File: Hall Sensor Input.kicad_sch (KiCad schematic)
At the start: 2 parts

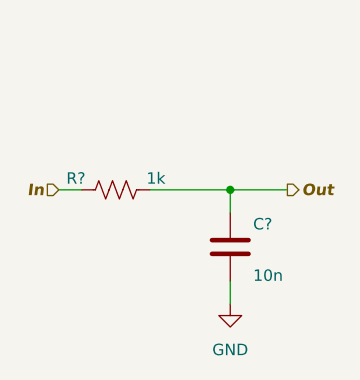
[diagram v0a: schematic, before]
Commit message: Ready for design review
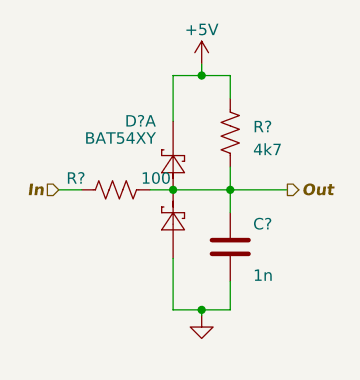
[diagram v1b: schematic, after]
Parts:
- added D?: BAT54XY, Package_TO_SOT_SMD:SOT-363_SC-70-6, symbol Diode:BAT54SW
- added R?: 4k7, Resistor_SMD:R_0402_1005Metric, symbol Device:R_US
- C?: value 10n -> 1n; DigiKey 490-4762-1-ND -> 490-GCM155R71H102KA37JCT-ND; LCSC (none) -> C1852263
- R?: value 1k -> 100; DigiKey 311-1.00KLRCT-ND -> 311-100JRCT-ND; LCSC (none) -> C106233
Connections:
- net GND: now also D?.1 (A)
- net Out: now also D?.6 (COM), R?.2
- new net +5V: D?.2 (K), R?.1

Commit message: Update
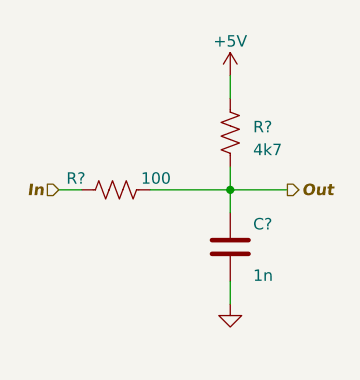
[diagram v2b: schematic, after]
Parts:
- removed D?: BAT54XY, Package_TO_SOT_SMD:SOT-363_SC-70-6, symbol Diode:BAT54SW
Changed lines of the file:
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@@
   (junction (at 146.05 101.6) (diameter 0) (color 0 0 0 0)
   )
-  (junction (at 139.7 101.6) (diameter 0) (color 0 0 0 0)
-  )
-  (junction (at 142.875 114.935) (diameter 0) (color 0 0 0 0)
-  )
-  (junction (at 142.875 88.9) (diameter 0) (color 0 0 0 0)
-  )
-  (wire (pts (xy 139.7 93.98) (xy 139.7 88.9))
-    (stroke (width 0) (type default))
-  )
-  (wire (pts (xy 142.875 114.935) (xy 142.875 115.57))
-    (stroke (width 0) (type default))
-  )
-  (wire (pts (xy 142.875 114.935) (xy 146.05 114.935))
-    (stroke (width 0) (type default))
-  )
-  (wire (pts (xy 146.05 114.935) (xy 146.05 111.76))
-    (stroke (width 0) (type default))
-  )
-  (wire (pts (xy 139.7 114.935) (xy 142.875 114.935))
+  (wire (pts (xy 146.05 114.3) (xy 146.05 111.76))
     (stroke (width 0) (type default))
   )
@@
     (stroke (width 0) (type default))
   )
-  (wire (pts (xy 139.7 109.22) (xy 139.7 114.935))
-    (stroke (width 0) (type default))
-  )
   (wire (pts (xy 146.05 99.06) (xy 146.05 101.6))
     (stroke (width 0) (type default))
   )
-  (wire (pts (xy 142.875 88.9) (xy 146.05 88.9))
-    (stroke (width 0) (type default))
-  )
   (wire (pts (xy 127 101.6) (xy 129.54 101.6))
     (stroke (width 0) (type default))
   )
-  (wire (pts (xy 137.16 101.6) (xy 139.7 101.6))
-    (stroke (width 0) (type default))
-  )
-  (wire (pts (xy 142.875 87.63) (xy 142.875 88.9))
+  (wire (pts (xy 137.16 101.6) (xy 146.05 101.6))
     (stroke (width 0) (type default))
   )
@@
     (stroke (width 0) (type default))
   )
-  (wire (pts (xy 139.7 88.9) (xy 142.875 88.9))
-    (stroke (width 0) (type default))
-  )
   (wire (pts (xy 146.05 88.9) (xy 146.05 91.44))
-    (stroke (width 0) (type default))
-  )
-  (wire (pts (xy 139.7 101.6) (xy 146.05 101.6))
     (stroke (width 0) (type default))
   )
@@
           (reference "C63") (unit 1)
         )
-        (path "/6b38a626-de8c-4b2d-bc76-3a02bc823a86/719c509b-8ff9-4083-837d-a3024db7e531"
-          (reference "C64") (unit 1)
-        )
-      )
-    )
-  )
-  (symbol (lib_id "power:GND") (at 142.875 115.57 0) (unit 1)
+      )
+    )
+  )
+  (symbol (lib_id "power:GND") (at 146.05 114.3 0) (unit 1)
     (in_bom yes) (on_board yes) (dnp no) (fields_autoplaced)
-    (property "Reference" "#PWR02" (at 142.875 121.92 0)
-      (effects (font (size 1.27 1.27)) hide)
-    )
-    (property "Value" "GND" (at 142.875 120.65 0)
-      (effects (font (size 1.27 1.27)) hide)
-    )
-    (property "Footprint" "" (at 142.875 115.57 0)
-      (effects (font (size 1.27 1.27)) hide)
-    )
-    (property "Datasheet" "" (at 142.875 115.57 0)
+    (property "Reference" "#PWR02" (at 146.05 120.65 0)
+      (effects (font (size 1.27 1.27)) hide)
+    )
+    (property "Value" "GND" (at 146.05 119.38 0)
+      (effects (font (size 1.27 1.27)) hide)
+    )
+    (property "Footprint" "" (at 146.05 114.3 0)
+      (effects (font (size 1.27 1.27)) hide)
+    )
+    (property "Datasheet" "" (at 146.05 114.3 0)
       (effects (font (size 1.27 1.27)) hide)
     )
@@
         (path "/6b38a626-de8c-4b2d-bc76-3a02bc823a86/a05ea58c-77e1-4772-b7c7-450b1547e96e"
           (reference "#PWR06") (unit 1)
-        )
-        (path "/6b38a626-de8c-4b2d-bc76-3a02bc823a86/719c509b-8ff9-4083-837d-a3024db7e531"
-          (reference "#PWR08") (unit 1)
         )
       )
@@
           (reference "R?") (unit 1)
         )
-        (path "/6b38a626-de8c-4b2d-bc76-3a02bc823a86/3c576bdf-2a9b-47b5-bf2f-8d65e4282c90"
-          (reference "R?") (unit 1)
-        )
         (path "/6b38a626-de8c-4b2d-bc76-3a02bc823a86/9e0a8a8b-b0ec-4703-8f8c-5ea275317857"
           (reference "R12") (unit 1)
@@
           (reference "R16") (unit 1)
         )
-        (path "/6b38a626-de8c-4b2d-bc76-3a02bc823a86/719c509b-8ff9-4083-837d-a3024db7e531"
-          (reference "R18") (unit 1)
-        )
-      )
-    )
-  )
-  (symbol (lib_id "Diode:BAT54SW") (at 139.7 101.6 90) (unit 1)
-    (in_bom yes) (on_board yes) (dnp no)
-    (property "Reference" "D?" (at 137.795 93.98 90)
-      (effects (font (size 1.27 1.27)) (justify left))
-    )
-    (property "Value" "BAT54XY" (at 137.795 95.885 90)
-      (effects (font (size 1.27 1.27)) (justify left))
-    )
-    (property "Footprint" "Package_TO_SOT_SMD:SOT-363_SC-70-6" (at 143.51 101.6 0)
-      (effects (font (size 1.27 1.27)) (justify left) hide)
-    )
-    (property "Datasheet" "https://assets.nexperia.com/documents/data-sheet/BAT54W_SER.pdf" (at 143.51 101.6 0)
-      (effects (font (size 1.27 1.27)) hide)
-    )
-    (property "LCSC" "C282367" (at 139.7 101.6 0)
-      (effects (font (size 1.27 1.27)) hide)
-    )
-    (property "DigiKey" "1727-3571-1-ND" (at 139.7 101.6 0)
-      (effects (font (size 1.27 1.27)) hide)
-    )
-    (pin "1")
-    (pin "2")
-    (pin "6")
-    (pin "3")
-    (pin "4")
-    (pin "5")
-    (instances
-      (project "ECE4760 Motor Driver"
-        (path "/6b38a626-de8c-4b2d-bc76-3a02bc823a86"
-          (reference "D?") (unit 1)
-        )
-        (path "/6b38a626-de8c-4b2d-bc76-3a02bc823a86/9895140f-573d-481d-a8a6-67e4fef141c0"
-          (reference "D?") (unit 1)
-        )
-        (path "/6b38a626-de8c-4b2d-bc76-3a02bc823a86/299487ec-ee2d-43f4-ae82-35783d2e6b45"
-          (reference "D?") (unit 2)
-        )
-        (path "/6b38a626-de8c-4b2d-bc76-3a02bc823a86/5fa307ae-0220-4647-a069-86a82689cac4"
-          (reference "D?") (unit 1)
-        )
-        (path "/6b38a626-de8c-4b2d-bc76-3a02bc823a86/3c576bdf-2a9b-47b5-bf2f-8d65e4282c90"
-          (reference "D?") (unit 2)
-        )
-        (path "/6b38a626-de8c-4b2d-bc76-3a02bc823a86/9e0a8a8b-b0ec-4703-8f8c-5ea275317857"
-          (reference "D1") (unit 1)
-        )
-        (path "/6b38a626-de8c-4b2d-bc76-3a02bc823a86/cdc8f404-9c8e-42d0-adf1-2d432268a04d"
-          (reference "D1") (unit 2)
-        )
-        (path "/6b38a626-de8c-4b2d-bc76-3a02bc823a86/a05ea58c-77e1-4772-b7c7-450b1547e96e"
-          (reference "D2") (unit 1)
-        )
-        (path "/6b38a626-de8c-4b2d-bc76-3a02bc823a86/719c509b-8ff9-4083-837d-a3024db7e531"
-          (reference "D2") (unit 2)
-        )
-      )
-    )
-  )
-  (symbol (lib_id "power:+5V") (at 142.875 87.63 0) (unit 1)
+      )
+    )
+  )
+  (symbol (lib_id "power:+5V") (at 146.05 88.9 0) (unit 1)
     (in_bom yes) (on_board yes) (dnp no) (fields_autoplaced)
-    (property "Reference" "#PWR01" (at 142.875 91.44 0)
-      (effects (font (size 1.27 1.27)) hide)
-    )
-    (property "Value" "+5V" (at 142.875 83.82 0)
+    (property "Reference" "#PWR01" (at 146.05 92.71 0)
+      (effects (font (size 1.27 1.27)) hide)
+    )
+    (property "Value" "+5V" (at 146.05 85.09 0)
       (effects (font (size 1.27 1.27)))
     )
-    (property "Footprint" "" (at 142.875 87.63 0)
-      (effects (font (size 1.27 1.27)) hide)
-    )
-    (property "Datasheet" "" (at 142.875 87.63 0)
+    (property "Footprint" "" (at 146.05 88.9 0)
+      (effects (font (size 1.27 1.27)) hide)
+    )
+    (property "Datasheet" "" (at 146.05 88.9 0)
       (effects (font (size 1.27 1.27)) hide)
     )
@@
         (path "/6b38a626-de8c-4b2d-bc76-3a02bc823a86/a05ea58c-77e1-4772-b7c7-450b1547e96e"
           (reference "#PWR05") (unit 1)
-        )
-        (path "/6b38a626-de8c-4b2d-bc76-3a02bc823a86/719c509b-8ff9-4083-837d-a3024db7e531"
-          (reference "#PWR07") (unit 1)
         )
       )
@@
           (reference "R17") (unit 1)
         )
-        (path "/6b38a626-de8c-4b2d-bc76-3a02bc823a86/719c509b-8ff9-4083-837d-a3024db7e531"
-          (reference "R19") (unit 1)
-        )
-      )
+      )

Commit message: Boards ordered!
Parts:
- C?: LCSC C1852263 -> C277522
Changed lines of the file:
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@@
       (effects (font (size 1.27 1.27)) hide)
     )
-    (property "LCSC" "C1852263" (at 146.05 107.95 0)
+    (property "LCSC" "C277522" (at 146.05 107.95 0)
       (effects (font (size 1.27 1.27)) hide)
     )
@@
         )
         (path "/6b38a626-de8c-4b2d-bc76-3a02bc823a86/9e0a8a8b-b0ec-4703-8f8c-5ea275317857"
-          (reference "C61") (unit 1)
+          (reference "C43") (unit 1)
         )
         (path "/6b38a626-de8c-4b2d-bc76-3a02bc823a86/cdc8f404-9c8e-42d0-adf1-2d432268a04d"
-          (reference "C62") (unit 1)
+          (reference "C44") (unit 1)
         )
         (path "/6b38a626-de8c-4b2d-bc76-3a02bc823a86/a05ea58c-77e1-4772-b7c7-450b1547e96e"
-          (reference "C63") (unit 1)
+          (reference "C45") (unit 1)
         )
       )
@@
   (symbol (lib_id "power:GND") (at 146.05 114.3 0) (unit 1)
     (in_bom yes) (on_board yes) (dnp no) (fields_autoplaced)
-    (property "Reference" "#PWR02" (at 146.05 120.65 0)
+    (property "Reference" "#PWR072" (at 146.05 120.65 0)
       (effects (font (size 1.27 1.27)) hide)
     )
@@
       (project "ECE4760 Motor Driver"
         (path "/6b38a626-de8c-4b2d-bc76-3a02bc823a86/9e0a8a8b-b0ec-4703-8f8c-5ea275317857"
-          (reference "#PWR02") (unit 1)
+          (reference "#PWR072") (unit 1)
         )
         (path "/6b38a626-de8c-4b2d-bc76-3a02bc823a86/cdc8f404-9c8e-42d0-adf1-2d432268a04d"
-          (reference "#PWR04") (unit 1)
+          (reference "#PWR074") (unit 1)
         )
         (path "/6b38a626-de8c-4b2d-bc76-3a02bc823a86/a05ea58c-77e1-4772-b7c7-450b1547e96e"
-          (reference "#PWR06") (unit 1)
+          (reference "#PWR076") (unit 1)
         )
       )
@@
         )
         (path "/6b38a626-de8c-4b2d-bc76-3a02bc823a86/9e0a8a8b-b0ec-4703-8f8c-5ea275317857"
-          (reference "R12") (unit 1)
+          (reference "R13") (unit 1)
         )
         (path "/6b38a626-de8c-4b2d-bc76-3a02bc823a86/cdc8f404-9c8e-42d0-adf1-2d432268a04d"
-          (reference "R14") (unit 1)
+          (reference "R15") (unit 1)
         )
         (path "/6b38a626-de8c-4b2d-bc76-3a02bc823a86/a05ea58c-77e1-4772-b7c7-450b1547e96e"
-          (reference "R16") (unit 1)
+          (reference "R17") (unit 1)
         )
       )
@@
   (symbol (lib_id "power:+5V") (at 146.05 88.9 0) (unit 1)
     (in_bom yes) (on_board yes) (dnp no) (fields_autoplaced)
-    (property "Reference" "#PWR01" (at 146.05 92.71 0)
+    (property "Reference" "#PWR071" (at 146.05 92.71 0)
       (effects (font (size 1.27 1.27)) hide)
     )
@@
       (project "ECE4760 Motor Driver"
         (path "/6b38a626-de8c-4b2d-bc76-3a02bc823a86/9e0a8a8b-b0ec-4703-8f8c-5ea275317857"
-          (reference "#PWR01") (unit 1)
+          (reference "#PWR071") (unit 1)
         )
         (path "/6b38a626-de8c-4b2d-bc76-3a02bc823a86/cdc8f404-9c8e-42d0-adf1-2d432268a04d"
-          (reference "#PWR03") (unit 1)
+          (reference "#PWR073") (unit 1)
         )
         (path "/6b38a626-de8c-4b2d-bc76-3a02bc823a86/a05ea58c-77e1-4772-b7c7-450b1547e96e"
-          (reference "#PWR05") (unit 1)
+          (reference "#PWR075") (unit 1)
         )
       )
@@
         )
         (path "/6b38a626-de8c-4b2d-bc76-3a02bc823a86/9e0a8a8b-b0ec-4703-8f8c-5ea275317857"
-          (reference "R13") (unit 1)
+          (reference "R14") (unit 1)
         )
         (path "/6b38a626-de8c-4b2d-bc76-3a02bc823a86/cdc8f404-9c8e-42d0-adf1-2d432268a04d"
-          (reference "R15") (unit 1)
+          (reference "R16") (unit 1)
         )
         (path "/6b38a626-de8c-4b2d-bc76-3a02bc823a86/a05ea58c-77e1-4772-b7c7-450b1547e96e"
-          (reference "R17") (unit 1)
+          (reference "R18") (unit 1)
         )
       )
